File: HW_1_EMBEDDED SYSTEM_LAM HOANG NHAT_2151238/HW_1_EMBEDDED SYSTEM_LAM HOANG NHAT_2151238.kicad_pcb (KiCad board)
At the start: 2 copper layers, 68.6 x 53.3 mm, 20 parts

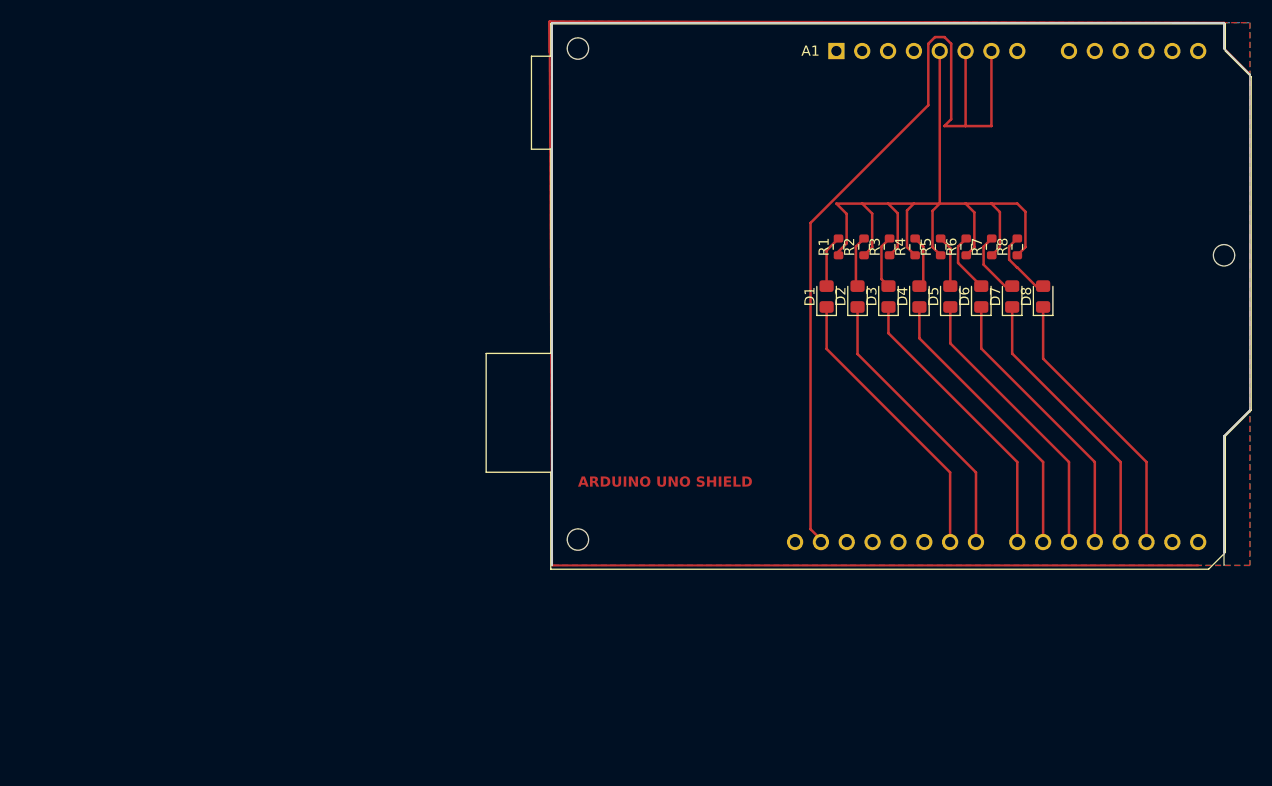
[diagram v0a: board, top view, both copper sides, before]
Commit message: Add files via upload
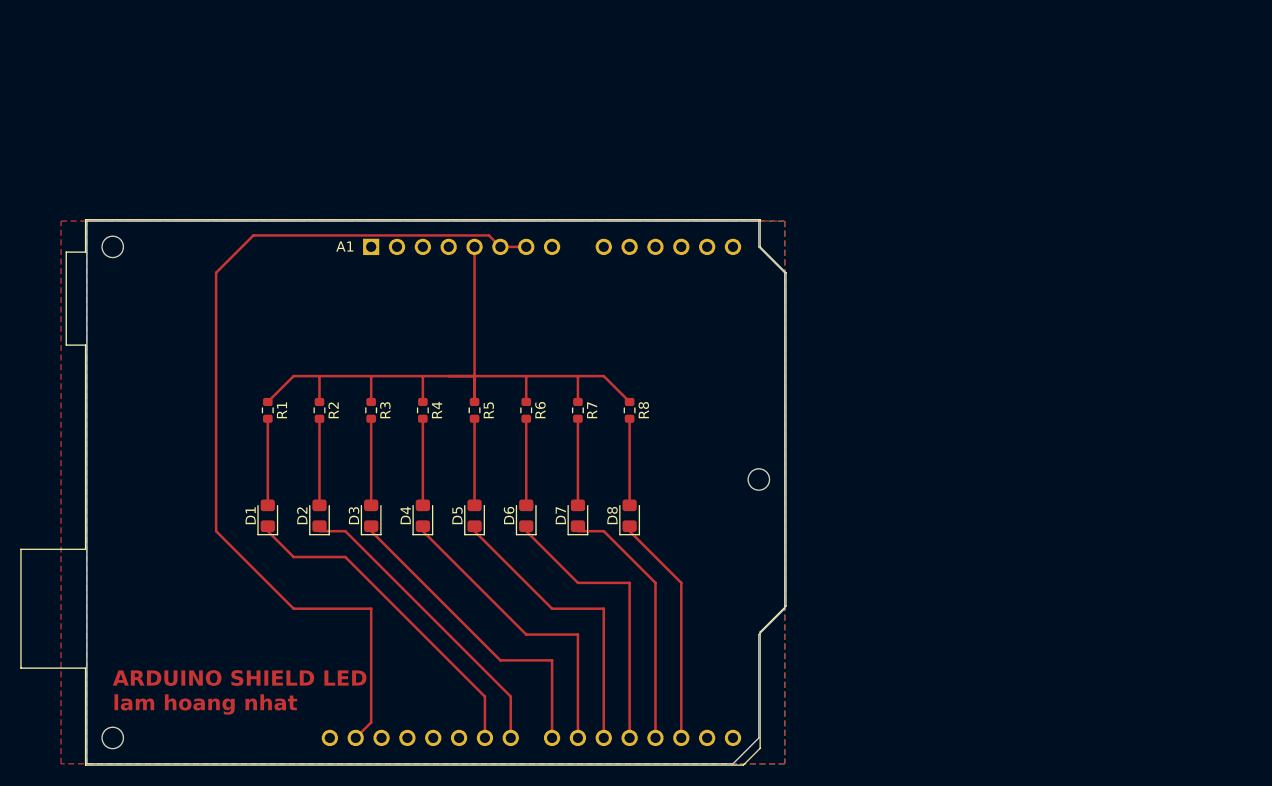
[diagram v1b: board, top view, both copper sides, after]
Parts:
- removed the REF** at (162.6, 55.9)
- removed the REF** at (162.6, 104.1)
- added REF**: MountingHole_2.1mm, MountingHole:MountingHole_2.1mm, F.Cu at (180.3, 98.2)
- added REF**: MountingHole_2.1mm, MountingHole:MountingHole_2.1mm, F.Cu at (116.8, 123.6)
- moved REF** 109.2 mm to (116.8, 75.4)
- moved D1 59.0 mm to (132.1, 101.8)
- moved R1 58.3 mm to (132.1, 91.4), turned to -90 degrees
- moved D2 57.1 mm to (137.2, 101.8)
- moved R2 55.9 mm to (137.2, 91.4), turned to -90 degrees
- moved D3 55.2 mm to (142.2, 101.8)
- moved R3 53.4 mm to (142.2, 91.4), turned to -90 degrees
- moved D4 53.3 mm to (147.3, 101.8)
- moved D5 51.5 mm to (152.4, 101.8)
- moved R4 51.0 mm to (147.3, 91.4), turned to -90 degrees
- moved D6 49.6 mm to (157.5, 101.8)
- moved A1 49.6 mm to (142.2, 75.4)
- moved R5 48.5 mm to (152.4, 91.4), turned to -90 degrees
- moved D7 47.8 mm to (162.6, 101.8)
- moved R6 46.1 mm to (157.5, 91.4), turned to -90 degrees
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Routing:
- net Net-(A1-+5V): track 79.1 -> 70.7 mm
- net Net-(A1-D2): track 27.1 -> 22.4 mm
- net GND: track 85.0 -> 89.6 mm
- net Net-(A1-D9): track 27.9 -> 32.1 mm
- net Net-(D5-A): track 5.07 -> 8.51 mm
- net Net-(D2-A): track 5.08 -> 8.51 mm
- net Net-(D1-A): track 5.16 -> 8.51 mm
- net Net-(D4-A): track 5.17 -> 8.51 mm
- net Net-(D3-A): track 5.30 -> 8.51 mm
- net Net-(A1-D7): track 28.1 -> 30.7 mm
- net Net-(D6-A): track 5.96 -> 8.51 mm
- net Net-(A1-D3): track 27.3 -> 25.0 mm
- net Net-(D7-A): track 6.59 -> 8.51 mm
- net Net-(A1-D8): track 27.7 -> 29.6 mm
- net Net-(A1-D6): track 27.9 -> 29.6 mm
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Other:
- outline, holes or cut-outs redrawn
- board text added: "ARDUINO SHIELD LED lam hoang nhat"
- board text removed: "ARDUINO UNO SHIELD"
